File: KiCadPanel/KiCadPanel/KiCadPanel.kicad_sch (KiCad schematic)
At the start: 64 parts, among them IC1 STP16CPC26PTR, IC10 STP16CPC26PTR, IC11 74HC4514PW,118, IC12 AP2281-3WG-7, IC13 AP2281-3WG-7, IC14 AP2281-3WG-7, IC15 AP2281-3WG-7, IC16 STP16CPC26PTR, IC17 AP2281-3WG-7, IC18 AP2281-3WG-7, IC19 AP2281-3WG-7, IC2 AP2281-3WG-7, IC20 AP2281-3WG-7, IC3 AP2281-3WG-7, IC4 AP2281-3WG-7, IC5 AP2281-3WG-7, IC6 AP2281-3WG-7, IC7 AP2281-3WG-7, IC8 AP2281-3WG-7, IC9 AP2281-3WG-7, J1 15-91-0100

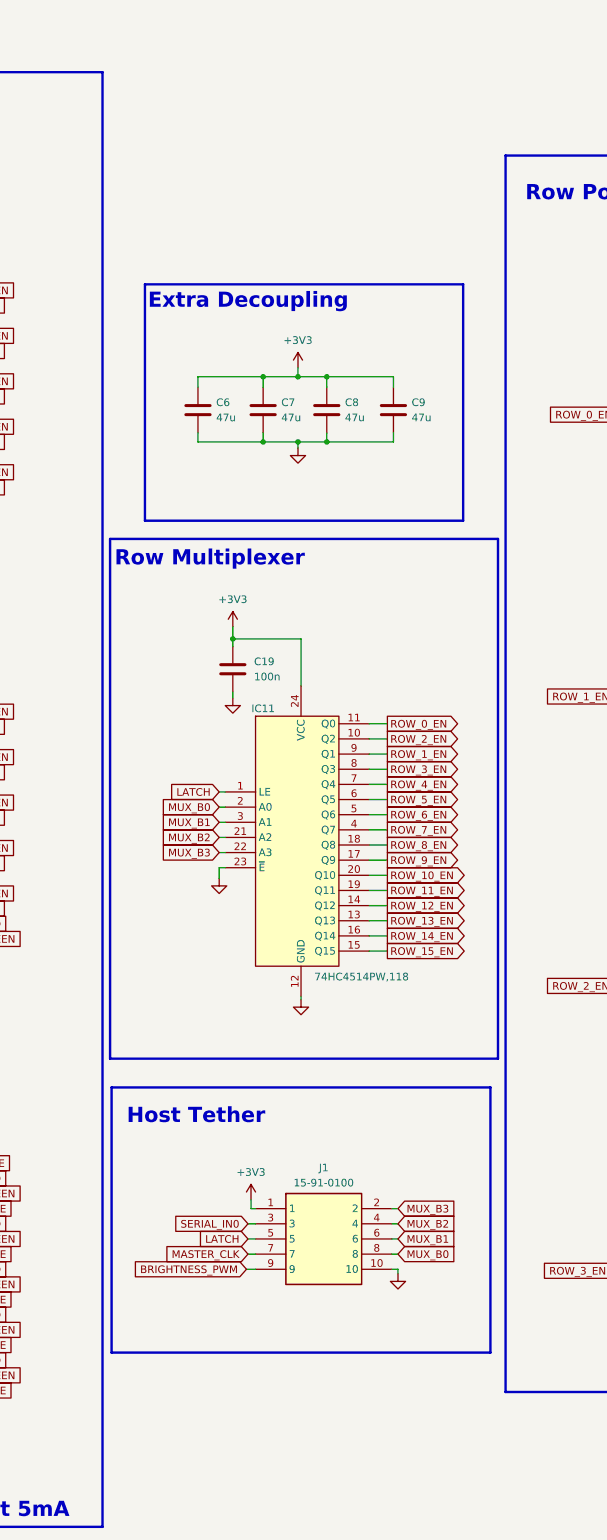
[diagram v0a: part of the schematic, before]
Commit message: Update for MTE
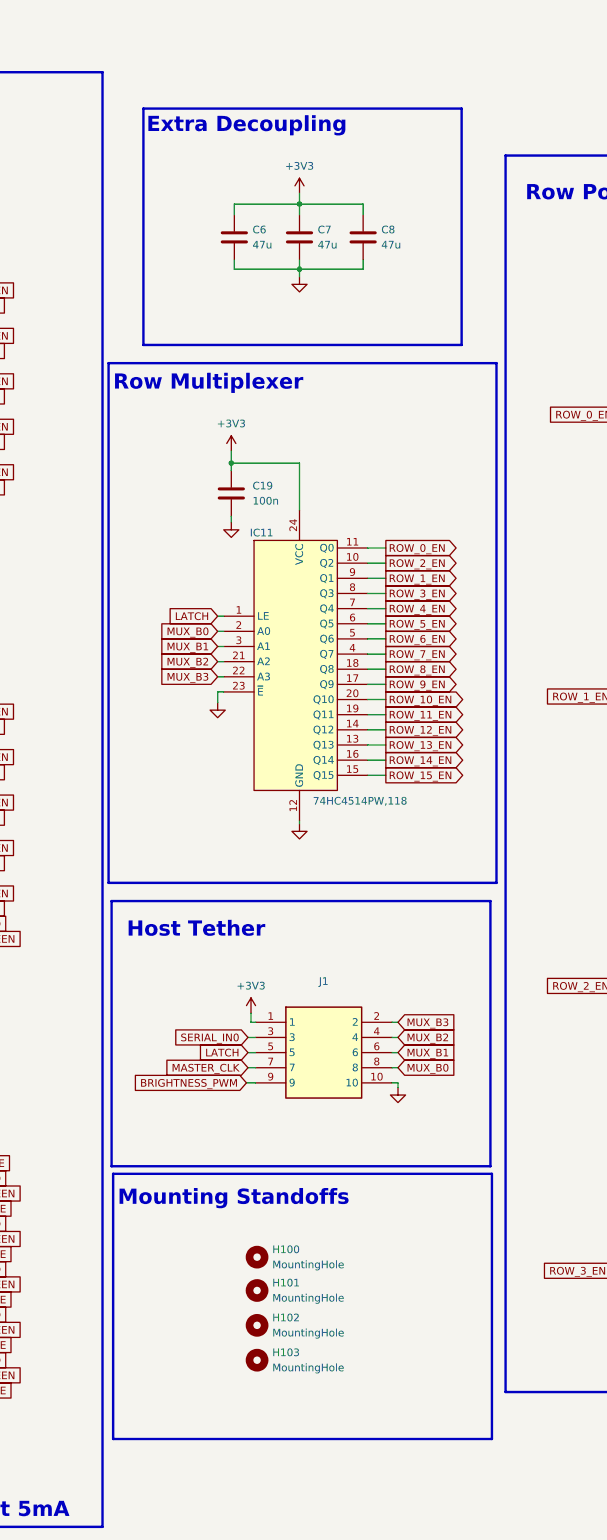
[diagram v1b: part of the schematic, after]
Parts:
- removed C9: 47u, Capacitor_SMD:C_1206_3216Metric, symbol Device:C
- added H100, H101, H102, H103: MountingHole, Mounting_Wuerth:Mounting_Wuerth_WA-SMSE-ExternalM3_H5mm_9771050360, symbol Mechanical:MountingHole
- J1: value 15-91-0100 -> ~; footprint SamacSys_Parts:FTSH10501FDVK -> LEDCubePanel:CNC_TECH_SMD_10POS
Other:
- note added: "Mounting Standoffs"
- moved on the sheet: C19, C6, C7, C8, IC11, J1
